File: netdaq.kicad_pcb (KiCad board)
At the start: 2 copper layers, 72 x 83 mm, 74 parts, among them J1 RJ45, U1 PIC32CK1025GC01100-I/4SB, U2 LAN8720A-CP, U3 MP6004GQ-P, U4 PD70100ILD-TR

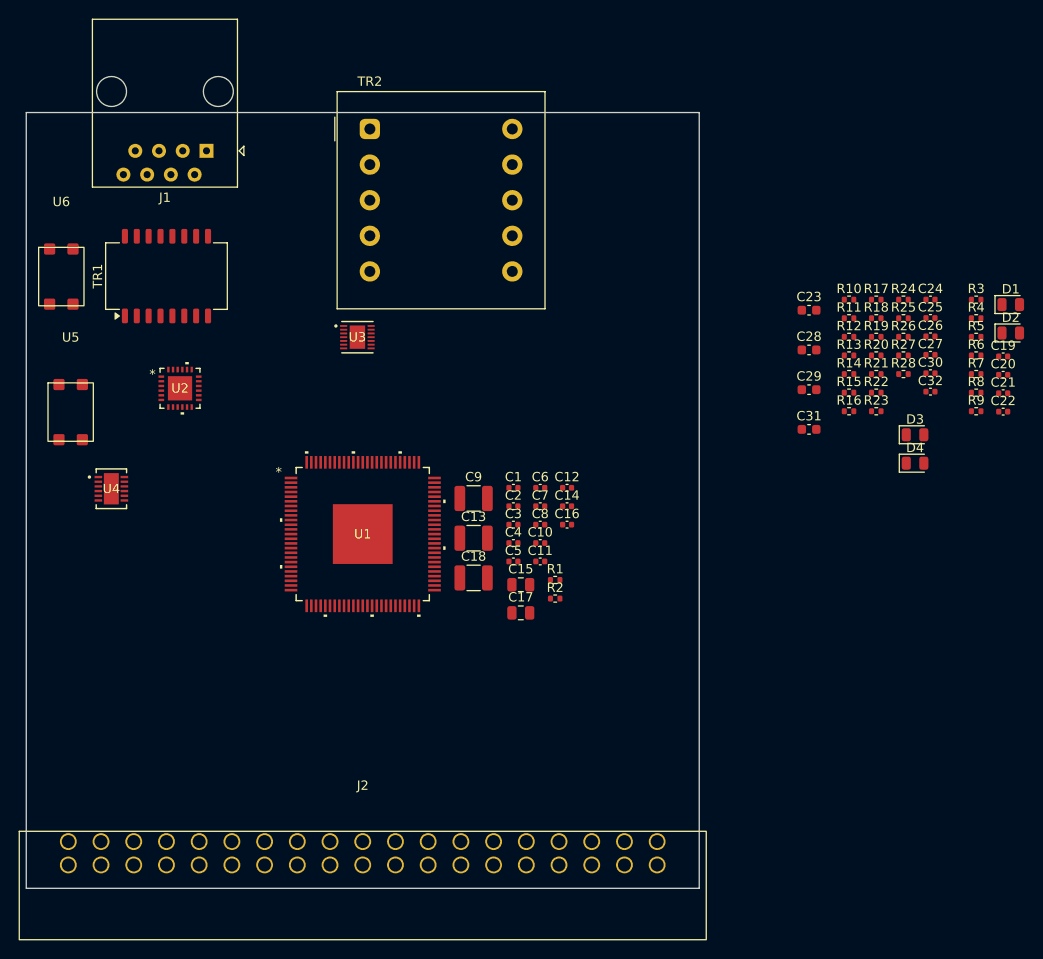
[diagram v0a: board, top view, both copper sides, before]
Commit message: stuff
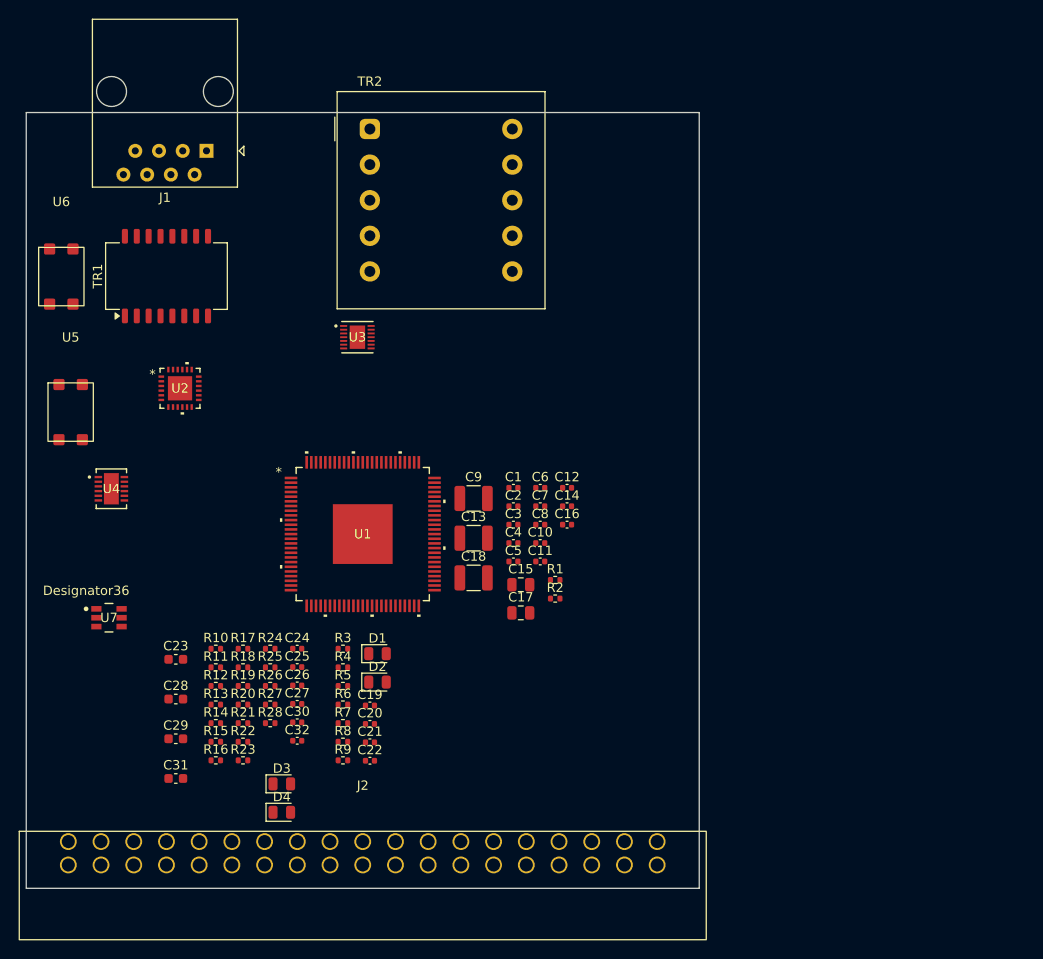
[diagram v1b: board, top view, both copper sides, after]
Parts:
- added U7: TPS62A01PDDCR, TPS62A01PDDCR:DDC0006A-MFG, F.Cu at (142.8, 116.0)
- moved C19 77.4 mm to (170.8, 125.4)
- moved C20 77.4 mm to (170.8, 127.4)
- moved C21 77.4 mm to (170.8, 129.4)
- moved C22 77.4 mm to (170.8, 131.3)
- moved C23 77.4 mm to (150.0, 120.5)
- moved C24 77.4 mm to (163.0, 119.4)
- moved C25 77.4 mm to (163.0, 121.3)
- moved C26 77.4 mm to (163.0, 123.3)
- moved C27 77.4 mm to (163.0, 125.3)
- moved C28 77.4 mm to (150.0, 124.8)
- moved C29 77.4 mm to (150.0, 129.0)
- moved C30 77.4 mm to (163.0, 127.2)
- moved C31 77.4 mm to (150.0, 133.2)
- moved C32 77.4 mm to (163.0, 129.2)
- moved D1 77.4 mm to (171.6, 119.9)
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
